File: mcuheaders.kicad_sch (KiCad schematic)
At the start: 4 parts, among them J1 Left_02x24, J2 Right_02x24, J20 Left Header, J4 Right Header

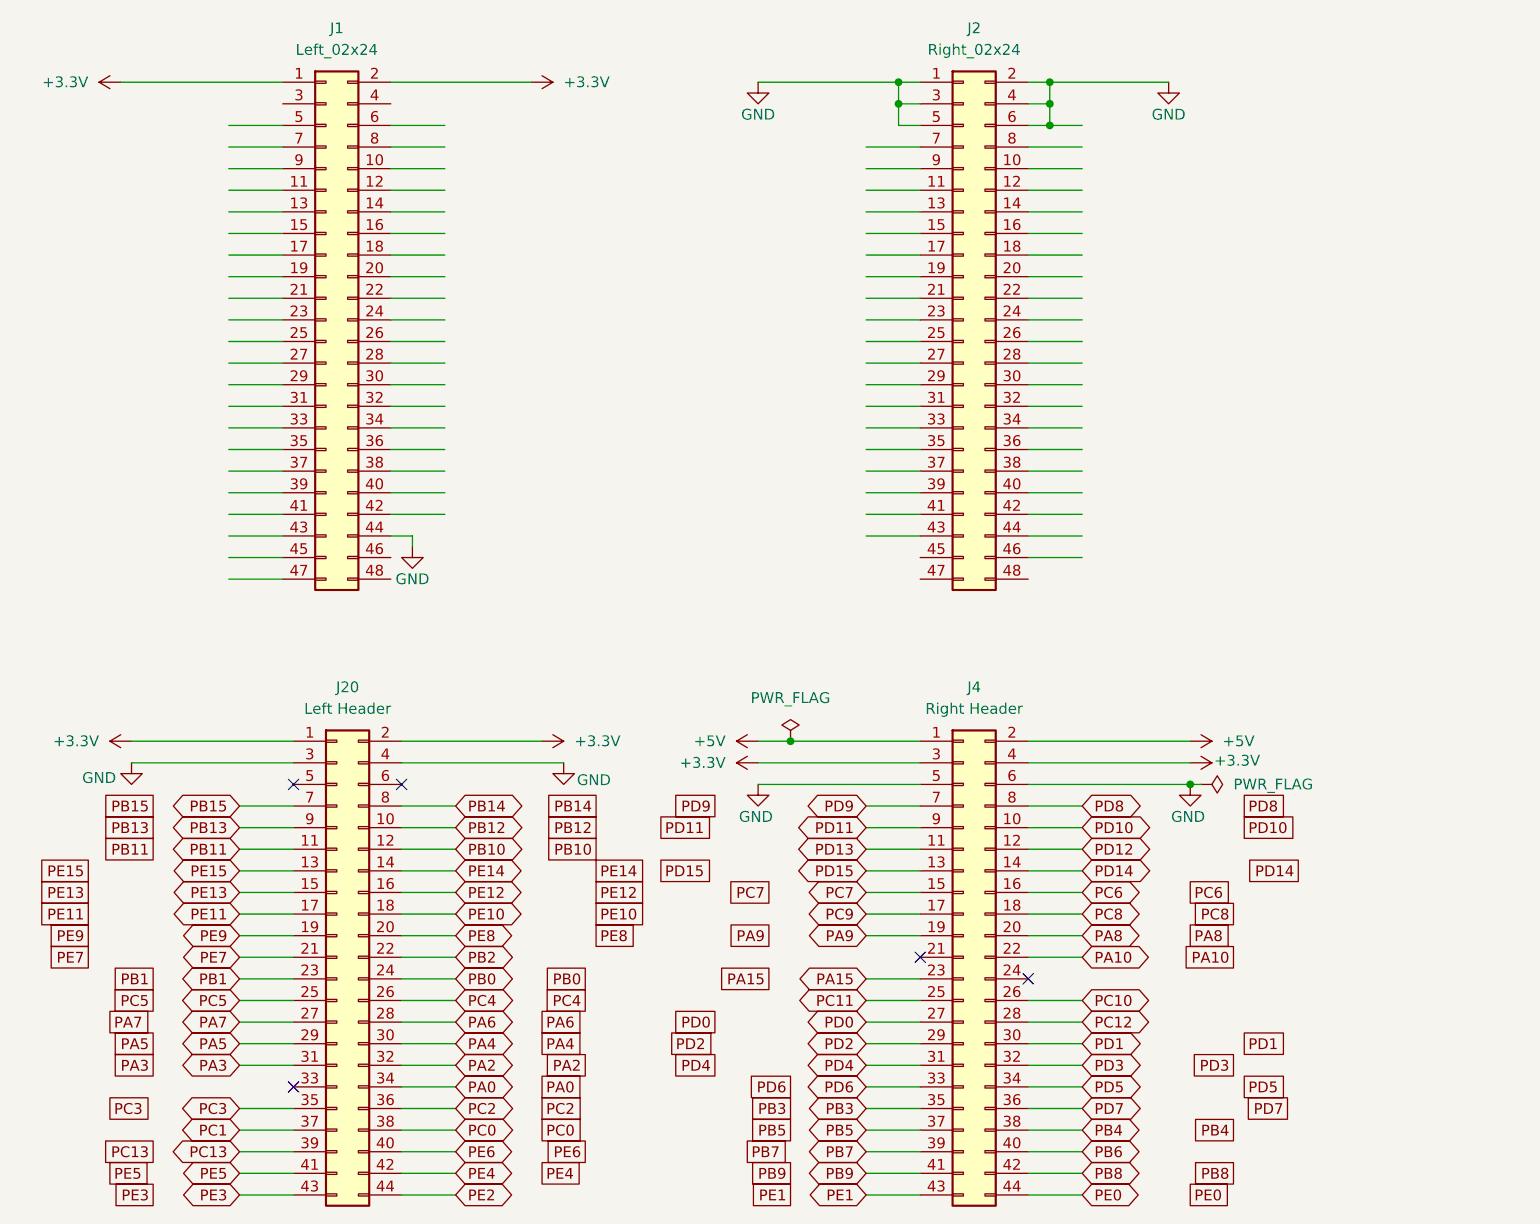
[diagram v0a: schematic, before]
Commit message: snapshot prior to clearing PCB
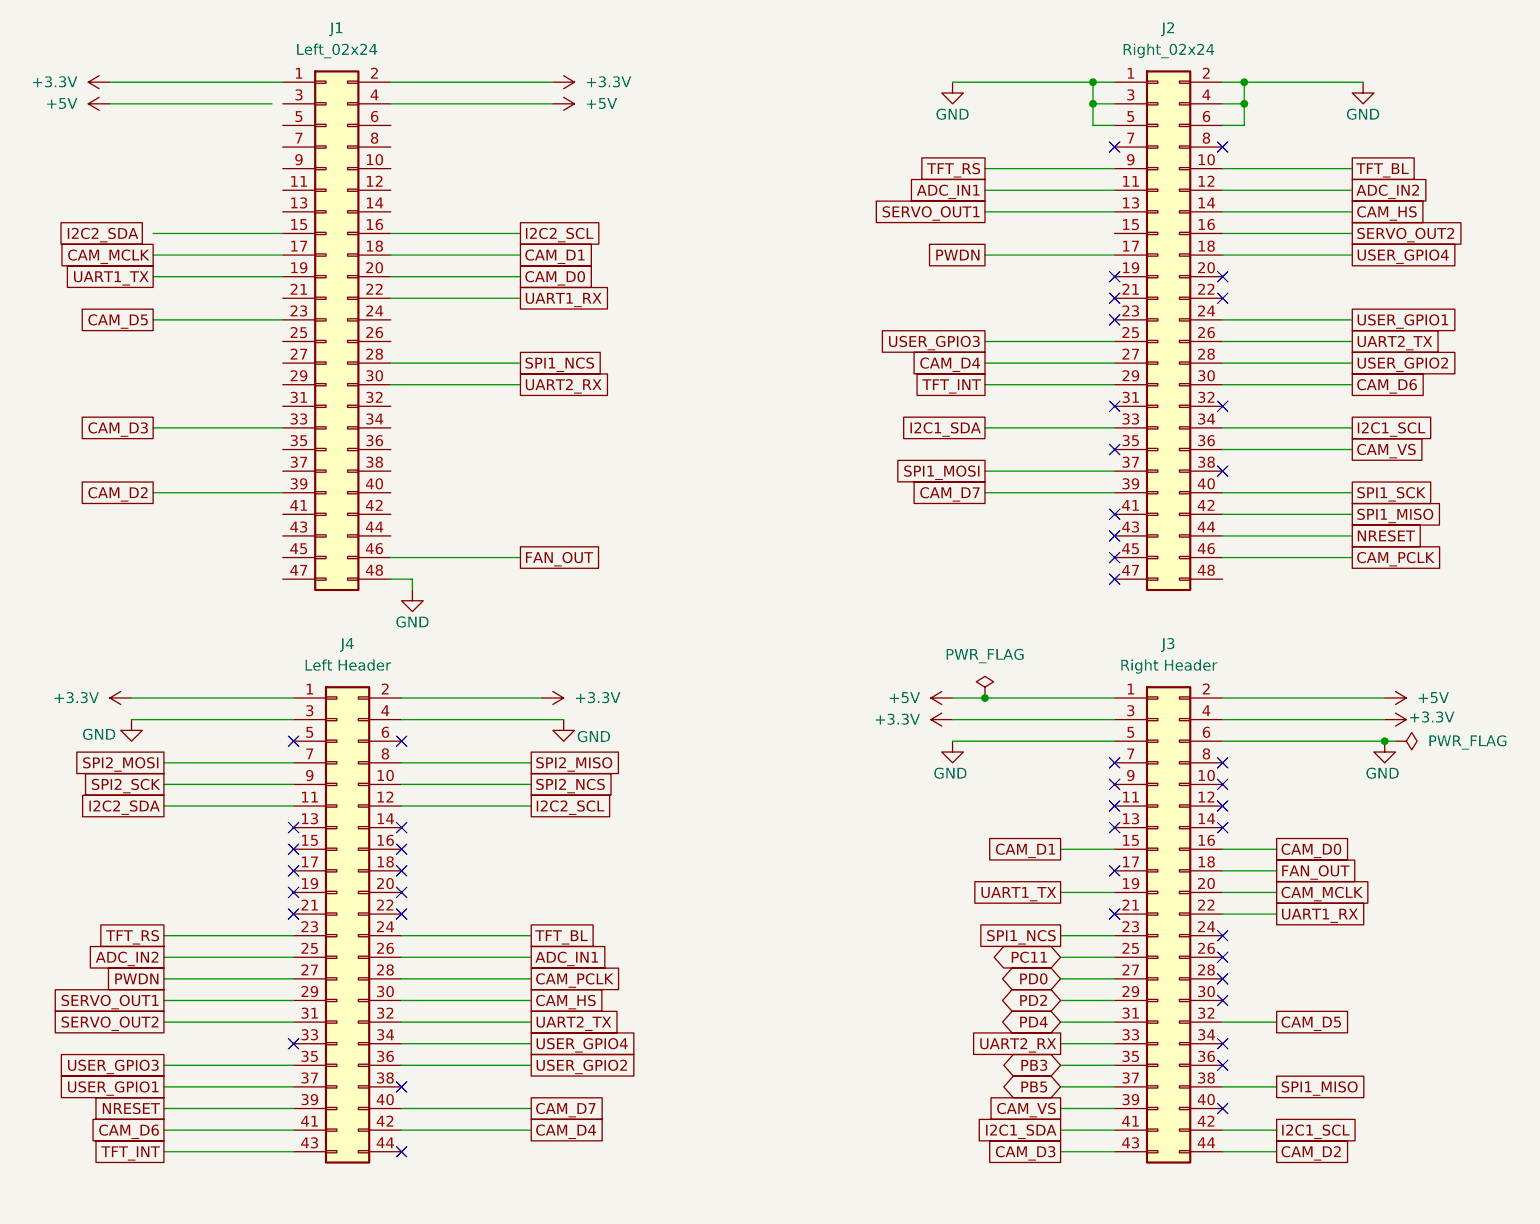
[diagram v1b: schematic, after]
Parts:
- J1, J2: footprint (none) -> Connector_PinHeader_2.54mm:PinHeader_2x24_P2.54mm_Vertical
- renumbered J4 to J3, J20 to J4
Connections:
- net PA0 is gone; now on net USER_GPIO4: J4.34 (Pin_34)
- net PA10 is gone; now on net UART1_RX: J3.22 (Pin_22)
- net PA15 is gone; now on net SPI1_NCS: J3.23 (Pin_23)
- net PA2 is gone; now on net UART2_TX: J4.32 (Pin_32)
- net PA3 is gone; now on net SERVO_OUT2: J4.31 (Pin_31)
- net PA4 is gone; now on net CAM_HS: J4.30 (Pin_30)
- net PA5 is gone; now on net SERVO_OUT1: J4.29 (Pin_29)
- net PA6 is gone; now on net CAM_PCLK: J4.28 (Pin_28)
- net PA7 is gone; now on net PWDN: J4.27 (Pin_27)
- net PA8 is gone; now on net CAM_MCLK: J3.20 (Pin_20)
- net PA9 is gone; now on net UART1_TX: J3.19 (Pin_19)
- net PB0 is gone; now on net TFT_BL: J4.24 (Pin_24)
- net PB1 is gone; now on net TFT_RS: J4.23 (Pin_23)
- net PB10 is gone; now on net I2C2_SCL: J4.12 (Pin_12)
- net PB4 is gone; now on net SPI1_MISO: J3.38 (Pin_38)
- net PB7 is gone; now on net CAM_VS: J3.39 (Pin_39)
- net PB8 is gone; now on net I2C1_SCL: J3.42 (Pin_42)
- net PB9 is gone; now on net I2C1_SDA: J3.41 (Pin_41)
- net PC1 is gone; now on net USER_GPIO1: J4.37 (Pin_37)
- net PC13 is gone; now on net NRESET: J4.39 (Pin_39)
- net PC2 is gone; now on net USER_GPIO2: J4.36 (Pin_36)
- net PC3 is gone; now on net USER_GPIO3: J4.35 (Pin_35)
- net PC4 is gone; now on net ADC_IN1: J4.26 (Pin_26)
- net PC5 is gone; now on net ADC_IN2: J4.25 (Pin_25)
- net PC6 is gone; now on net CAM_D0: J3.16 (Pin_16)
- net PC7 is gone; now on net CAM_D1: J3.15 (Pin_15)
- net PC8 is gone; now on net FAN_OUT: J3.18 (Pin_18)
- net PD3 is gone; now on net CAM_D5: J3.32 (Pin_32)
- net PD6 is gone; now on net UART2_RX: J3.33 (Pin_33)
- net PE0 is gone; now on net CAM_D2: J3.44 (Pin_44)
- net PE1 is gone; now on net CAM_D3: J3.43 (Pin_43)
- net PE3 is gone; now on net TFT_INT: J4.43 (Pin_43)
- net PE4 is gone; now on net CAM_D4: J4.42 (Pin_42)
- net PE5 is gone; now on net CAM_D6: J4.41 (Pin_41)
- net PE6 is gone; now on net CAM_D7: J4.40 (Pin_40)
- net +5V: now also J1.4 (Pin_4)
- net GND: now also J1.48 (Pin_48); no longer J1.44 (Pin_44)
- net TFT_BL: now reaches J2.10 (Pin_10)
- net ADC_IN1: now reaches J2.11 (Pin_11)
- net ADC_IN2: now reaches J2.12 (Pin_12)
- net SERVO_OUT1: now reaches J2.13 (Pin_13)
- net CAM_HS: now reaches J2.14 (Pin_14)
- net SERVO_OUT2: now reaches J2.16 (Pin_16)
- net PWDN: now reaches J2.17 (Pin_17)
- net USER_GPIO4: now reaches J2.18 (Pin_18)
- net USER_GPIO1: now reaches J2.24 (Pin_24)
- net USER_GPIO3: now reaches J2.25 (Pin_25)
- net UART2_TX: now reaches J2.26 (Pin_26)
- net CAM_D4: now reaches J2.27 (Pin_27)
- net USER_GPIO2: now reaches J2.28 (Pin_28)
- net TFT_INT: now reaches J2.29 (Pin_29)
- net CAM_D6: now reaches J2.30 (Pin_30)
- net I2C1_SDA: now reaches J2.33 (Pin_33)
- net I2C1_SCL: now reaches J2.34 (Pin_34)
- net CAM_VS: now reaches J2.36 (Pin_36)
- net SPI1_MOSI: now reaches J2.37 (Pin_37)
- net CAM_D7: now reaches J2.39 (Pin_39)
- net SPI1_SCK: now reaches J2.40 (Pin_40)
- net SPI1_MISO: now reaches J2.42 (Pin_42)
- net NRESET: now reaches J2.44 (Pin_44)
- net CAM_PCLK: now reaches J2.46 (Pin_46)
- net TFT_RS: now reaches J2.9 (Pin_9)
- net I2C2_SCL: now reaches J1.16 (Pin_16)
- net CAM_MCLK: now reaches J1.17 (Pin_17)
- net CAM_D1: now reaches J1.18 (Pin_18)
- net UART1_TX: now reaches J1.19 (Pin_19)
- net CAM_D0: now reaches J1.20 (Pin_20)
- net UART1_RX: now reaches J1.22 (Pin_22)
- net CAM_D5: now reaches J1.23 (Pin_23)
- net SPI1_NCS: now reaches J1.28 (Pin_28)
- net UART2_RX: now reaches J1.30 (Pin_30)
- net CAM_D3: now reaches J1.33 (Pin_33)
- net CAM_D2: now reaches J1.39 (Pin_39)
- net FAN_OUT: now reaches J1.46 (Pin_46)
- net PB11 renamed I2C2_SDA
- net PB12 renamed SPI2_NCS
- net PB13 renamed SPI2_SCK
- net PB14 renamed SPI2_MISO
- net PB15 renamed SPI2_MOSI
- net PB2: no longer names the net of J4.22 (Pin_22)
- net PB6: no longer names the net of J3.40 (Pin_40)
- net PC0: no longer names the net of J4.38 (Pin_38)
- net PC10: no longer names the net of J3.26 (Pin_26)
- net PC12: no longer names the net of J3.28 (Pin_28)
- net PC9: no longer names the net of J3.17 (Pin_17)
- net PD1: no longer names the net of J3.30 (Pin_30)
- net PD10: no longer names the net of J3.10 (Pin_10)
- net PD11: no longer names the net of J3.9 (Pin_9)
- net PD12: no longer names the net of J3.12 (Pin_12)
- net PD13: no longer names the net of J3.11 (Pin_11)
- net PD14: no longer names the net of J3.14 (Pin_14)
- net PD15: no longer names the net of J3.13 (Pin_13)
- net PD5: no longer names the net of J3.34 (Pin_34)
- net PD7: no longer names the net of J3.36 (Pin_36)
- net PD8: no longer names the net of J3.8 (Pin_8)
- net PD9: no longer names the net of J3.7 (Pin_7)
- net PE10: no longer names the net of J4.18 (Pin_18)
- net PE11: no longer names the net of J4.17 (Pin_17)
- net PE12: no longer names the net of J4.16 (Pin_16)
- net PE13: no longer names the net of J4.15 (Pin_15)
- net PE14: no longer names the net of J4.14 (Pin_14)
- net PE15: no longer names the net of J4.13 (Pin_13)
- net PE2: no longer names the net of J4.44 (Pin_44)
- net PE7: no longer names the net of J4.21 (Pin_21)
- net PE8: no longer names the net of J4.20 (Pin_20)
- net PE9: no longer names the net of J4.19 (Pin_19)
- no-connect marks 5 -> 47
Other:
- moved on the sheet: J2, J3, J4
